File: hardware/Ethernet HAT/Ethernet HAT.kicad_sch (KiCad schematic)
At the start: 42 parts, among them J1 RJ45_Amphenol_RJMG1BD3B8K1ANR, J2 1-84952-4, U1 W5500, Y1 Crystal_25MHz

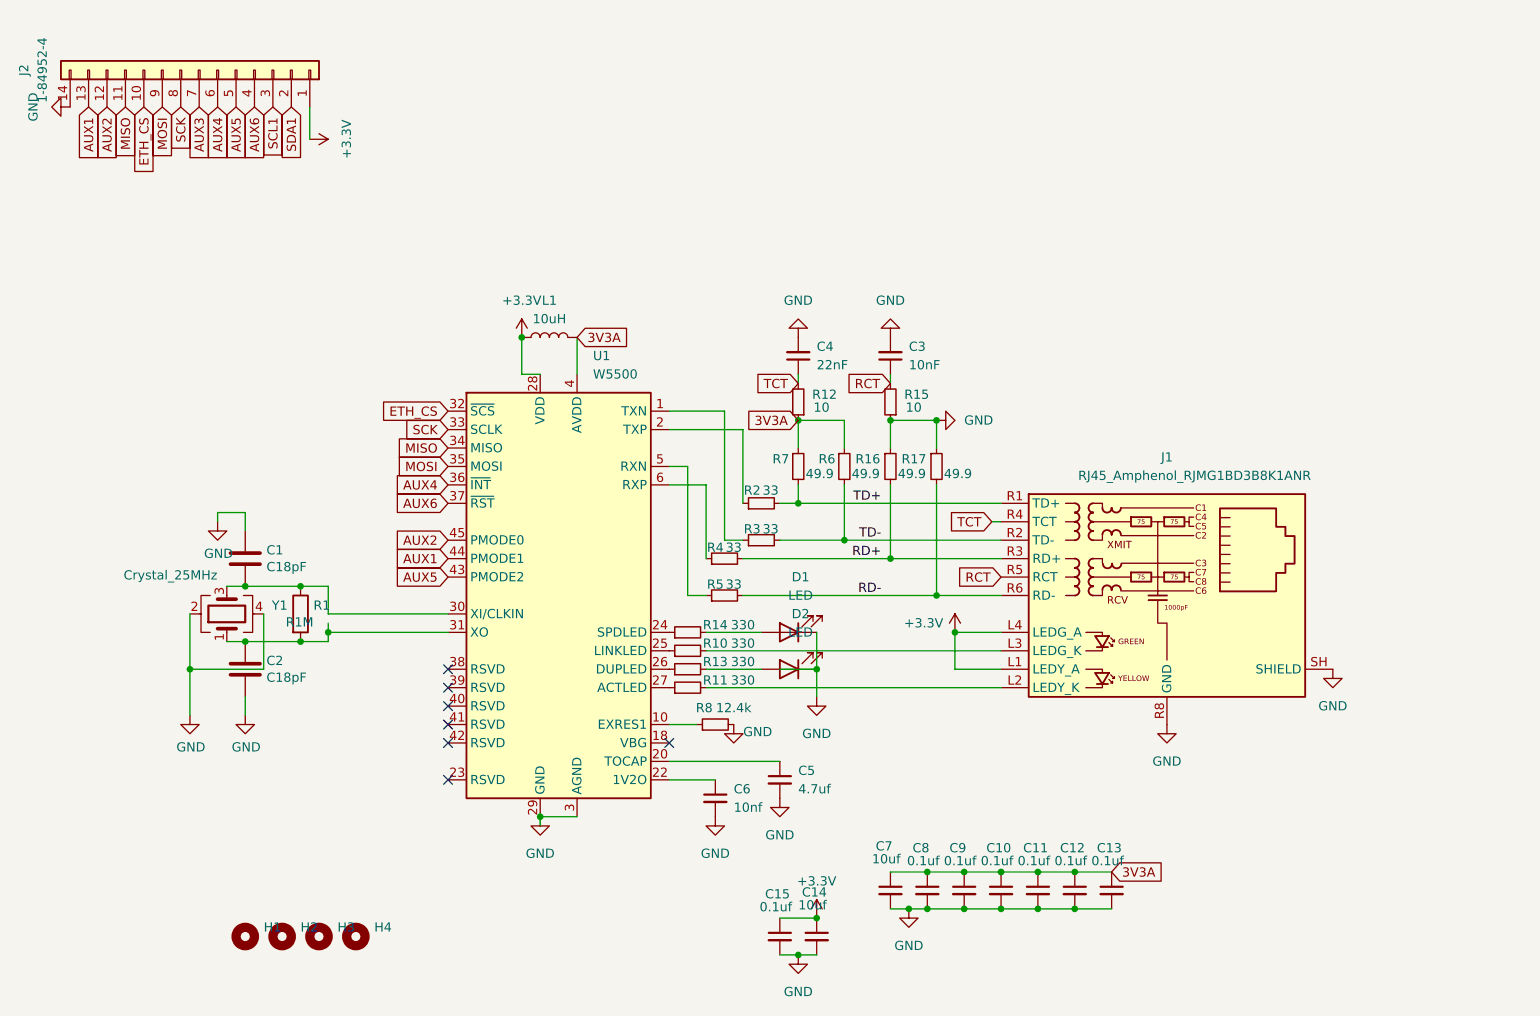
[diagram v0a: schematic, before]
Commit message: Ethernet HAT V1.2.0
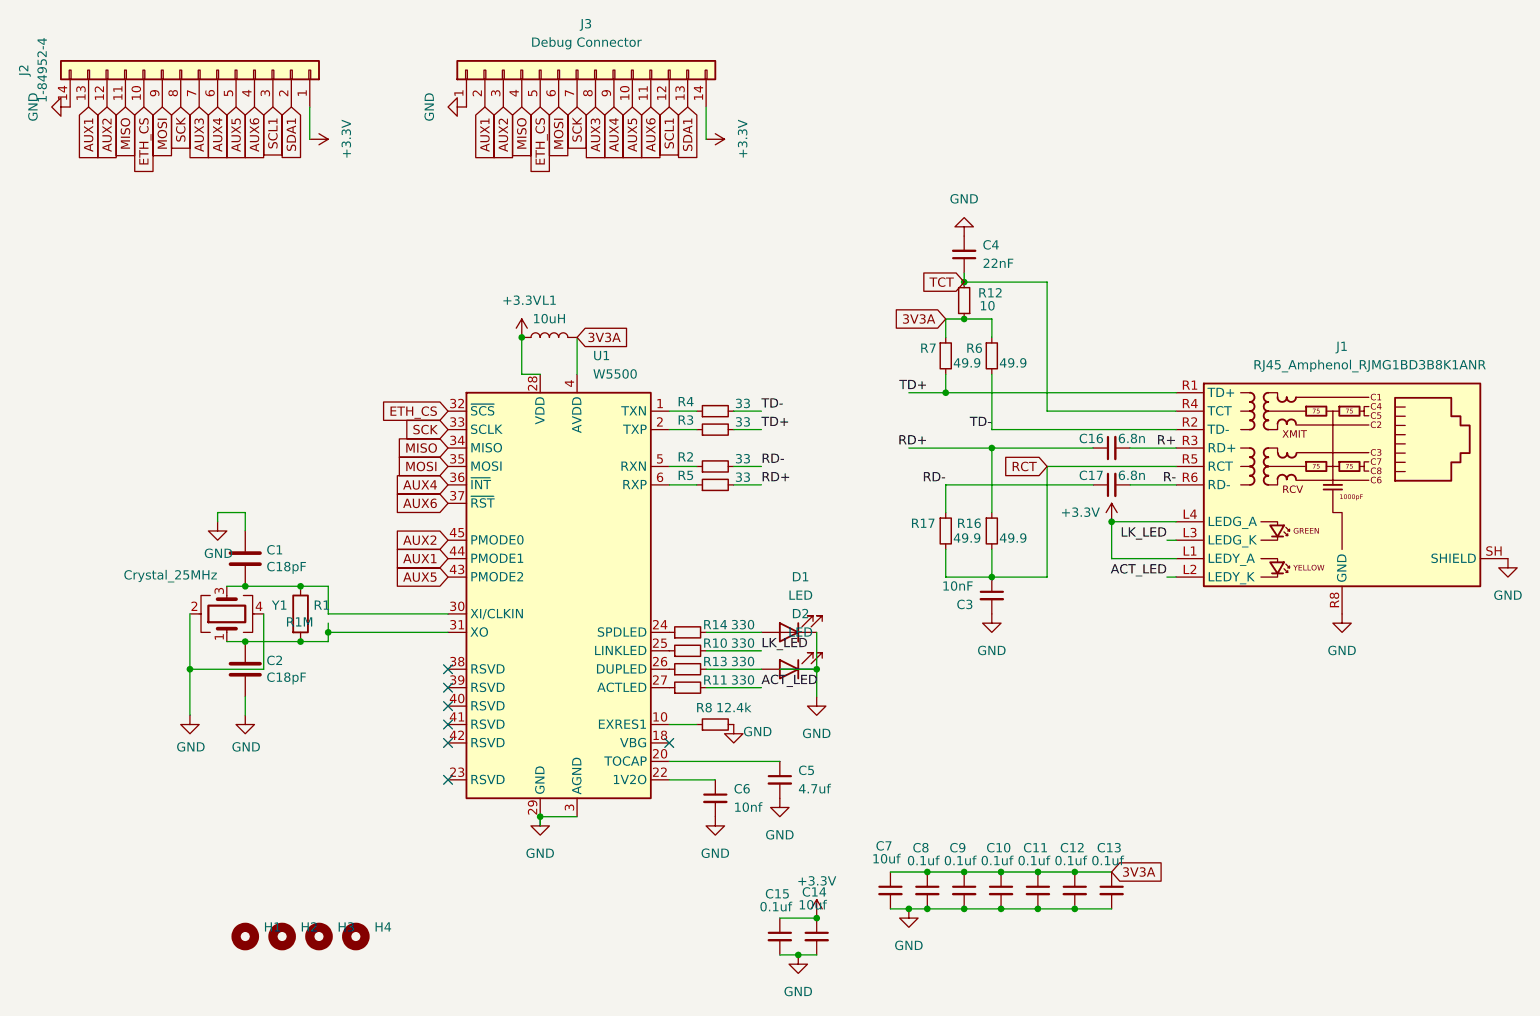
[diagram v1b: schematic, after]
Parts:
- removed R15: 10, Resistor_SMD:R_0402_1005Metric, symbol Device:R_Small
- added C16, C17: 6.8n, Capacitor_SMD:C_0402_1005Metric, symbol Device:C_Small
- added J3: Debug Connector, GE_Connector:Conn_01x14_Flat2.54, symbol Connector_Generic:Conn_01x14
- R8: footprint Resistor_SMD:R_0402_1005Metric -> Resistor_SMD:R_0603_1608Metric
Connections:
- net +3.3V: now also J3.14 (Pin_14)
- net AUX1: now also J3.2 (Pin_2)
- net AUX2: now also J3.3 (Pin_3)
- net AUX3: now also J3.8 (Pin_8)
- net AUX4: now also J3.9 (Pin_9)
- net AUX5: now also J3.10 (Pin_10)
- net AUX6: now also J3.11 (Pin_11)
- net ETH_CS: now also J3.5 (Pin_5)
- net GND: now also J3.1 (Pin_1); no longer R16.1, R17.1
- net MISO: now also J3.4 (Pin_4)
- net MOSI: now also J3.6 (Pin_6)
- net RCT: now also R16.2, R17.2
- net RD+: now also R16.1, R5.2, C16.1; no longer J1.R3 (RD+), R16.2, R4.2
- net RD-: now also R17.1, R2.2, C17.1; no longer J1.R6 (RD-), R17.2, R5.2
- net SCK: now also J3.7 (Pin_7)
- net SCL1: now also J3.12 (Pin_12)
- net SDA1: now also J3.13 (Pin_13)
- net TD+: now also R3.2; no longer R2.2
- net TD-: now also R4.2; no longer R3.2
- net at R2.1: now also U1.5 (RXN); no longer U1.2 (TXP)
- net ACT_LED: now reaches J1.L2 (LEDY_K), R11.2
- net LK_LED: now reaches J1.L3 (LEDG_K), R10.2
- net at U1.1 (TXN): now also R4.1; no longer R3.1
- net at R5.1: now also U1.6 (RXP); no longer U1.5 (RXN)
- new net: R3.1, U1.2 (TXP)
- new net R+: C16.2, J1.R3 (RD+)
- new net R-: C17.2, J1.R6 (RD-)
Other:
- moved on the sheet: C3, C4, J1, R12, R16, R17, R6, R7
